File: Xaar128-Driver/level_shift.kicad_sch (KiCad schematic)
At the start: 21 parts, among them Q1 DMN2075U, U10 74AHCT125, U5 TXB0104D, U6 TXB0104D, U7 TXB0104D, U8 74AHCT125, U9 74AHCT125

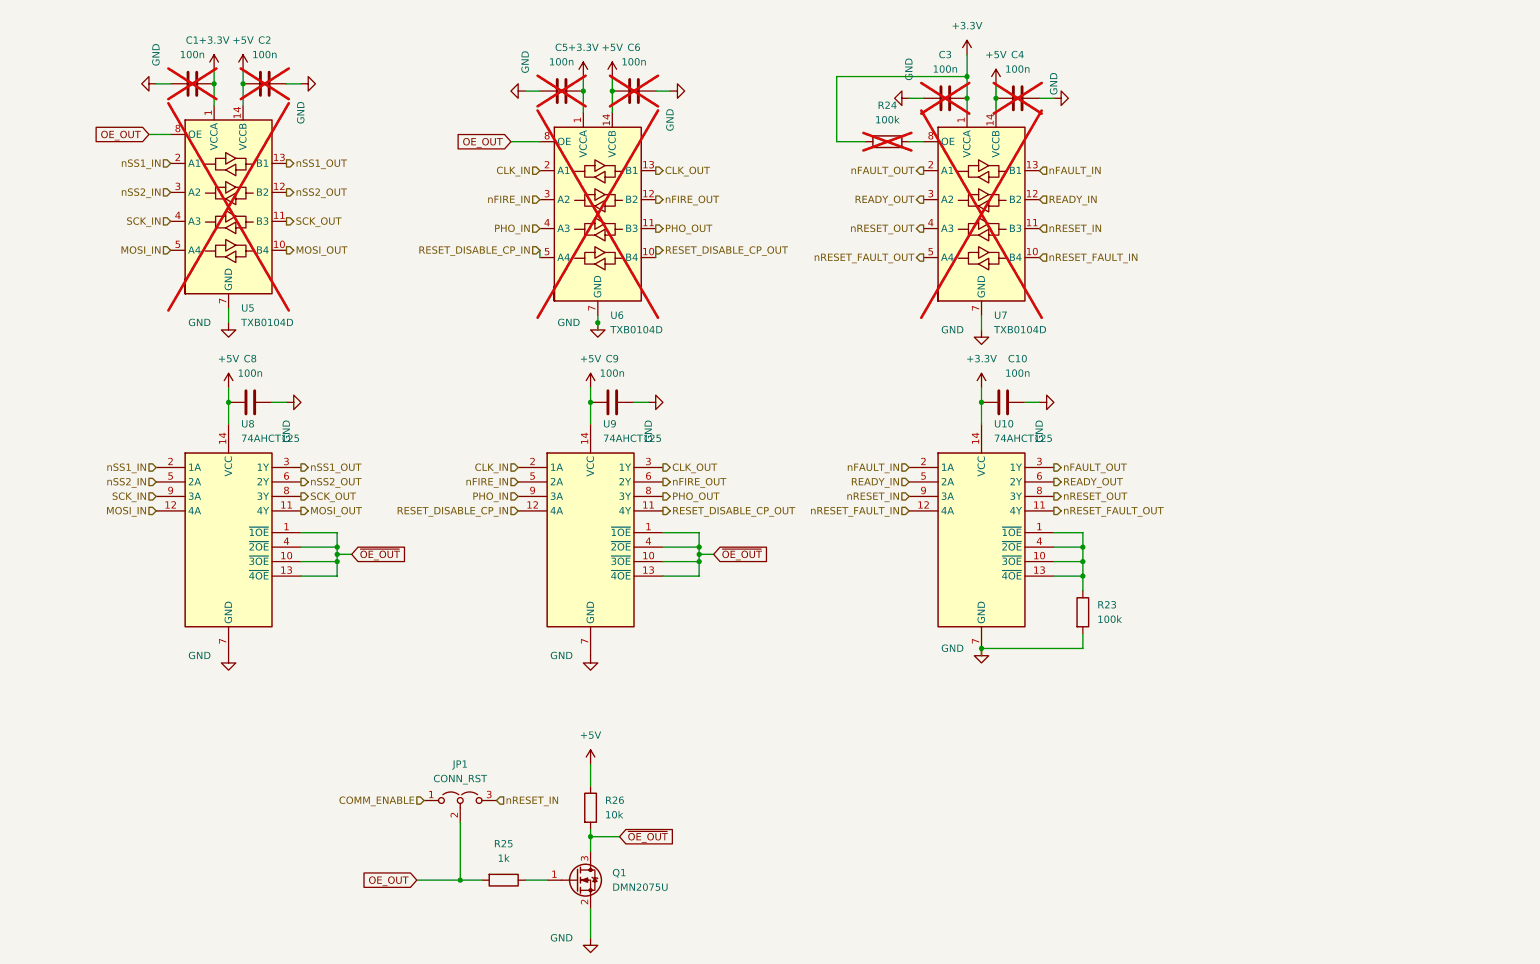
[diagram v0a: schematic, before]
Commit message: 5v monitoring
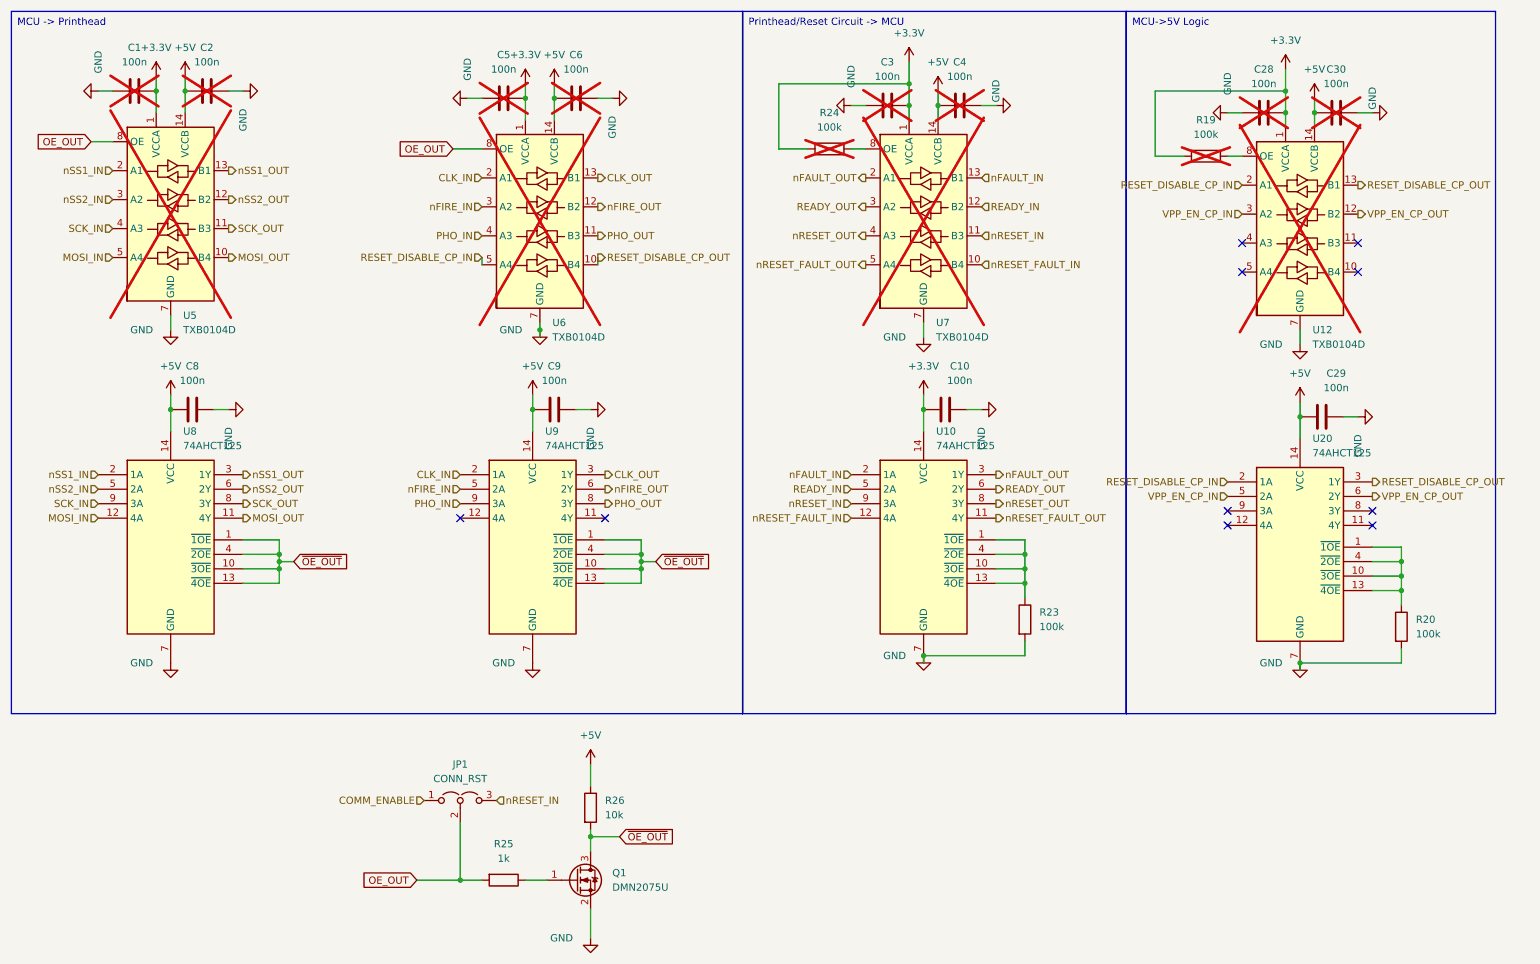
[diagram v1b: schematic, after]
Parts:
- added C28, C29, C30: 100n, symbol Device:C
- added R19, R20: 100k, symbol Device:R
- added U12: TXB0104D, Package_SO:SOIC-14_3.9x8.7mm_P1.27mm, symbol Logic_LevelTranslator:TXB0104D
- added U20: 74AHCT125, symbol Xaar_Driver:74AHCT125
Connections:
- net +3.3V: now also C28.2, R19.1, U12.1 (VCCA)
- net +5V: now also C29.2, C30.2, U12.14 (VCCB), U20.14 (VCC)
- net GND: now also C28.1, C29.1, C30.1, R20.2, U12.7 (GND), U20.7 (GND)
- net RESET_DISABLE_CP_IN: now also U12.2 (A1), U20.2 (1A); no longer U9.12 (4A)
- net RESET_DISABLE_CP_OUT: now also U12.13 (B1), U20.3 (1Y); no longer U9.11 (4Y)
- new net: R20.1, U20.1 (~{1OE}), U20.10 (~{3OE}), U20.13 (~{4OE}), U20.4 (~{2OE})
- new net: R19.2, U12.8 (OE)
- new net VPP_EN_CP_IN: U12.3 (A2), U20.5 (2A)
- new net VPP_EN_CP_OUT: U12.12 (B2), U20.6 (2Y)
- no-connect marks 0 -> 10
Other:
- moved on the sheet: C1, C10, C2, C3, C4, C5, C6, C8, C9, R23, R24, U10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
